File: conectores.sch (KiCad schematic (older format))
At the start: 31 parts, among them IC2 Corriente C, J5 TENSION

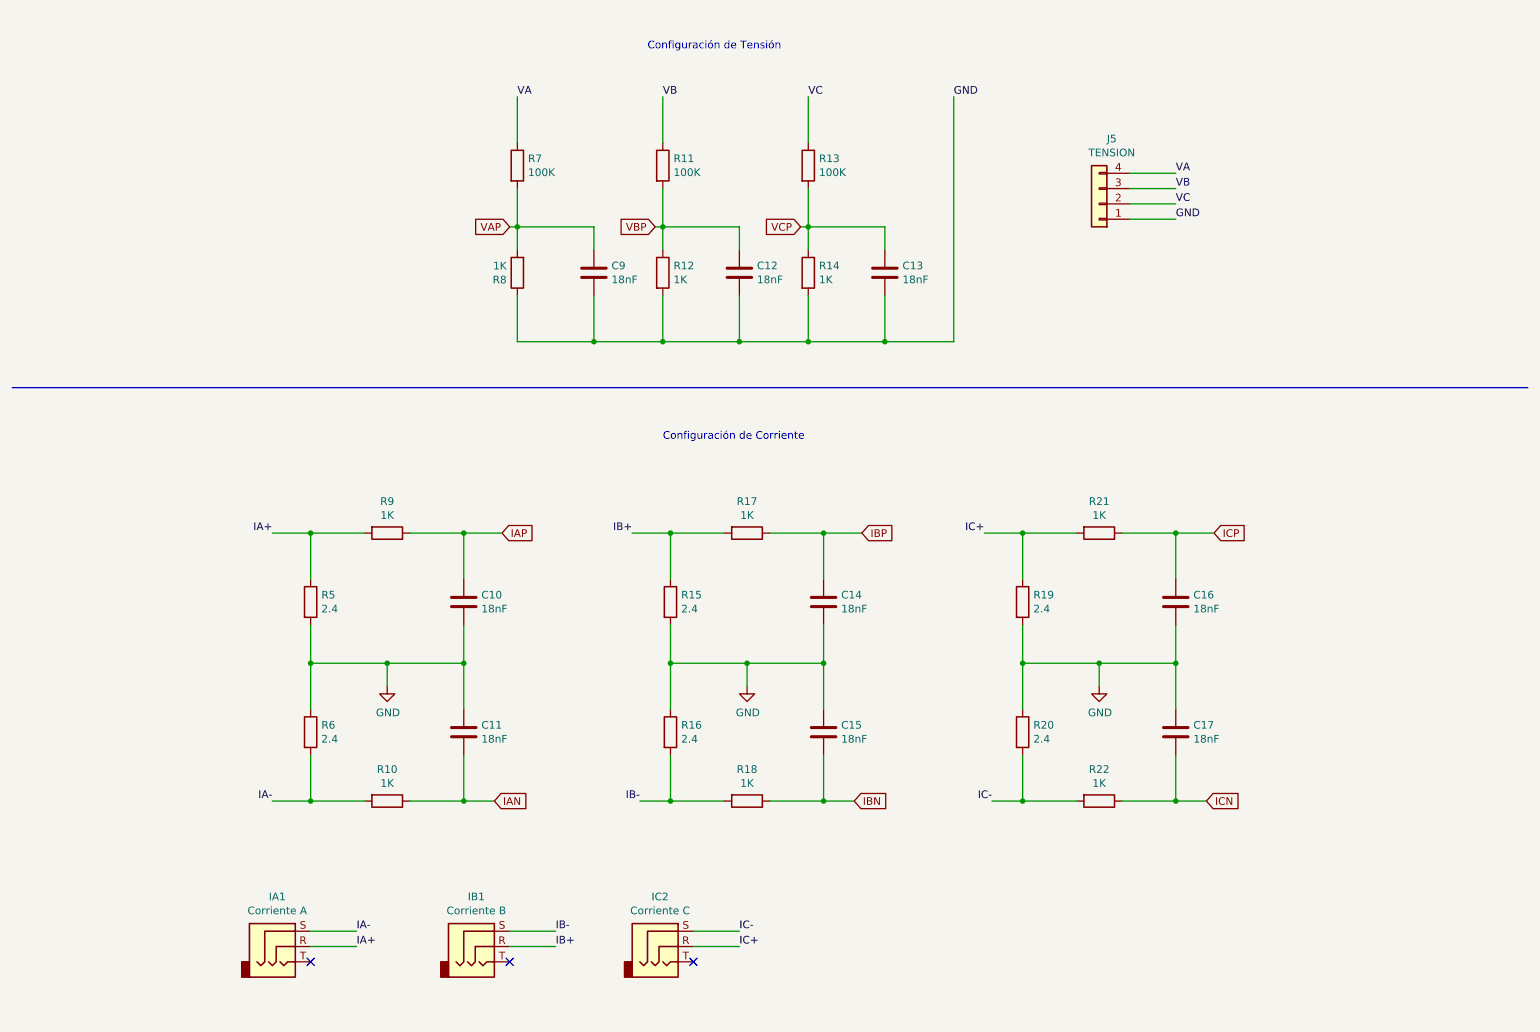
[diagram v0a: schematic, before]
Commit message: Add files via upload
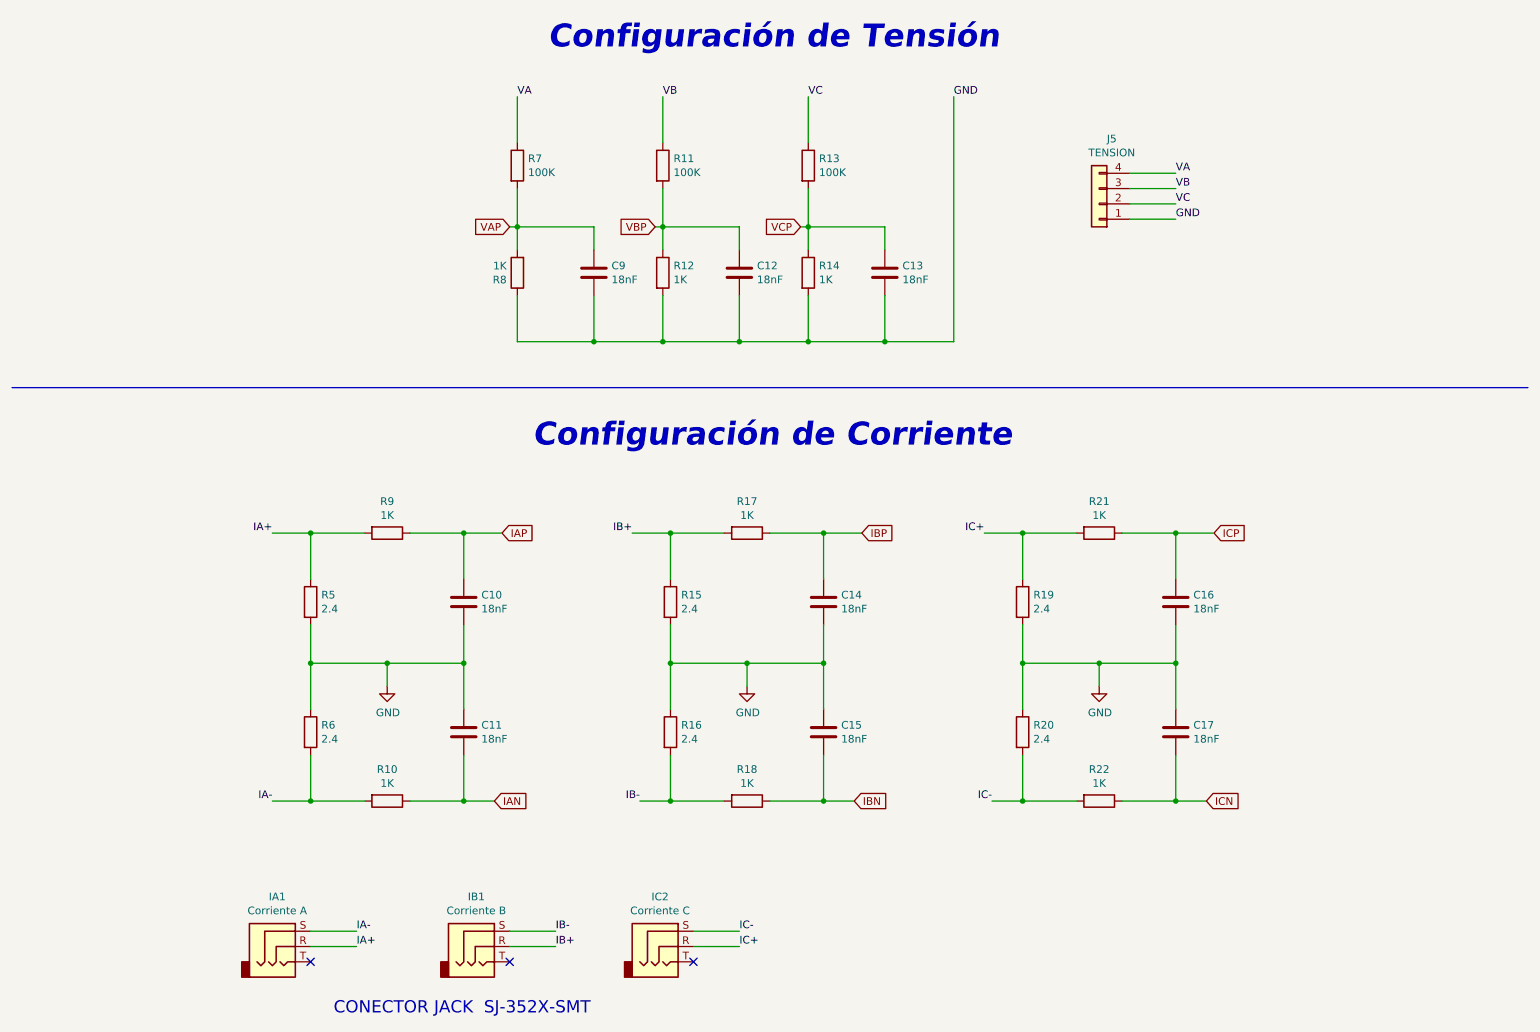
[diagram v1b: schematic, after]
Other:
- note added: "CONECTOR JACK SJ-352X-SMT"
- note added: "Configuración de Corriente"
- note removed: "Configuración de Corriente\n"
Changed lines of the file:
@@
 Wire Bus Line
 	750  3100 10650 3100
-Text Notes 4900 900  0    50   ~ 0
+Text Notes 4250 900  0    150  Italic 30
 Configuración de Tensión
-Text Notes 5000 3450 0    50   ~ 0
-Configuración de Corriente\n
 $Comp
 L Connector:AudioJack3 IA1
@@
 	1    0    0    -1
 $EndComp
+Text Notes 2850 7200 0    80   ~ 0
+CONECTOR JACK  SJ-352X-SMT
+Text Notes 4150 3500 0    150  Italic 30
+Configuración de Corriente
 $EndSCHEMATC
